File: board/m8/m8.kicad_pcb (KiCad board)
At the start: 2 copper layers, 50 x 25 mm, 11 parts, among them J1 program, SW1 B3F-4000, U1 CH32V003f4p6

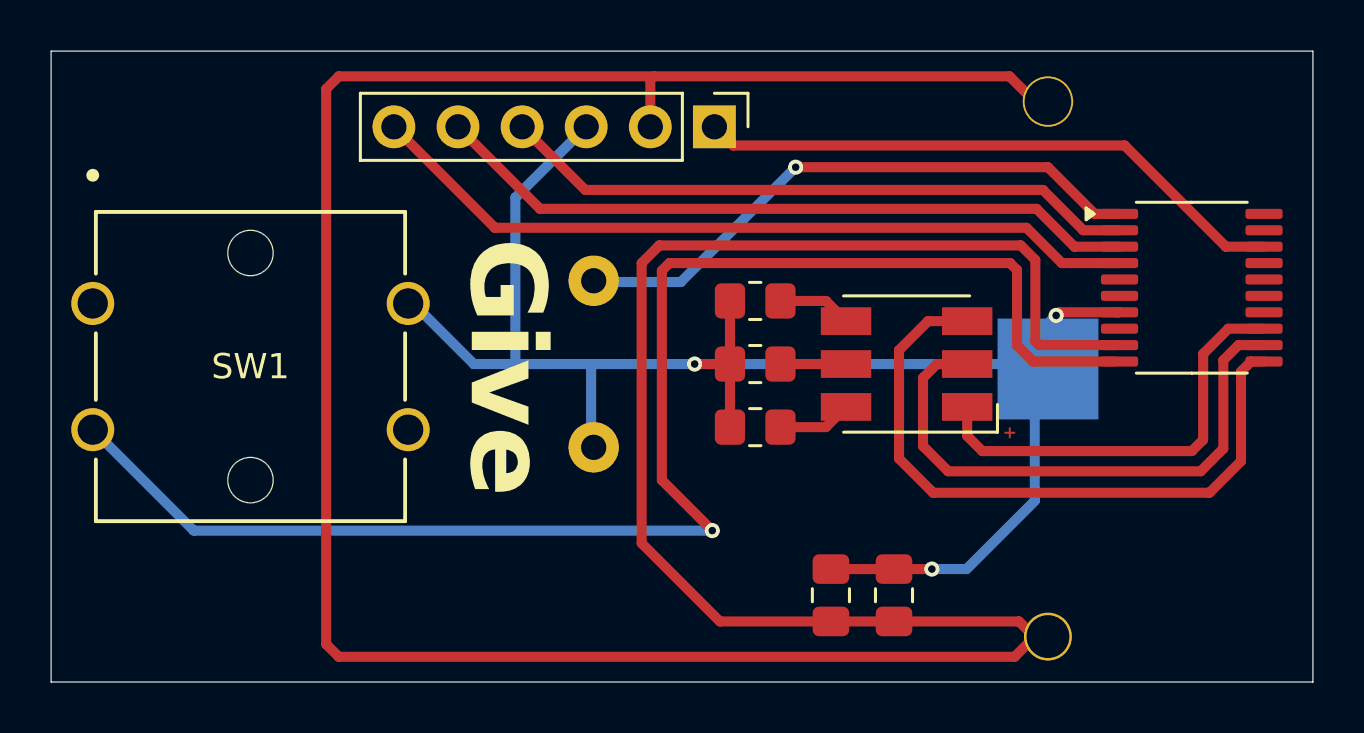
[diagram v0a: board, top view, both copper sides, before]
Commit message: rev2 with sugestions from Chip
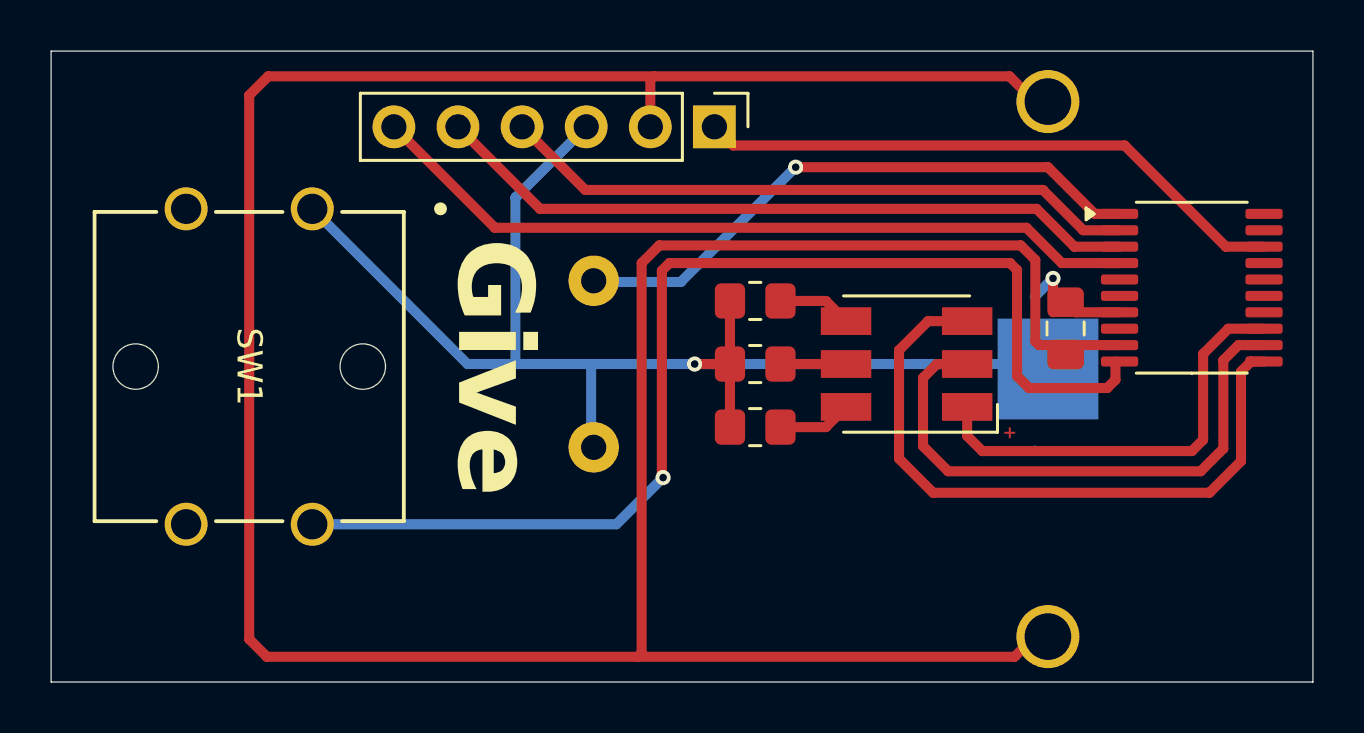
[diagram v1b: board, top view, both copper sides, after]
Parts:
- removed C2: 100n, Capacitor_SMD:C_0805_2012Metric_Pad1.18x1.45mm_HandSolder
- C1: value 10u -> 100n
- moved C1 12.6 mm to (159.8, 111.0)
- moved SW1 9.47 mm to (129.9, 106.2), turned to -90 degrees
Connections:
- SW1 pad 1: unconnected-(SW1-Pad1) -> GND
- SW1 pad 2: GND -> Net-(U1-PC0_T2CH3)
- SW1 pad 3: Net-(U1-PC0_T2CH3) -> unconnected-(SW1-Pad3)
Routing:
- net Net-(U1-PC0_T2CH3): track 59.4 -> 46.9 mm
- net GND: track 65.9 -> 56.6 mm, vias 3 -> 2
- net VCC: track 132.2 -> 125.9 mm
